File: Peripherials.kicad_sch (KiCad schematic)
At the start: 24 parts, among them J10 IDC_Cable_02x08, J6 Conn_01x02_Pin, J7 USB_C_Receptacle_USB2.0_14P, J8 USB_C_Receptacle_USB2.0_14P, Q1 NMOS, U5 USBLC6-2P6, U6 USBLC6-2P6

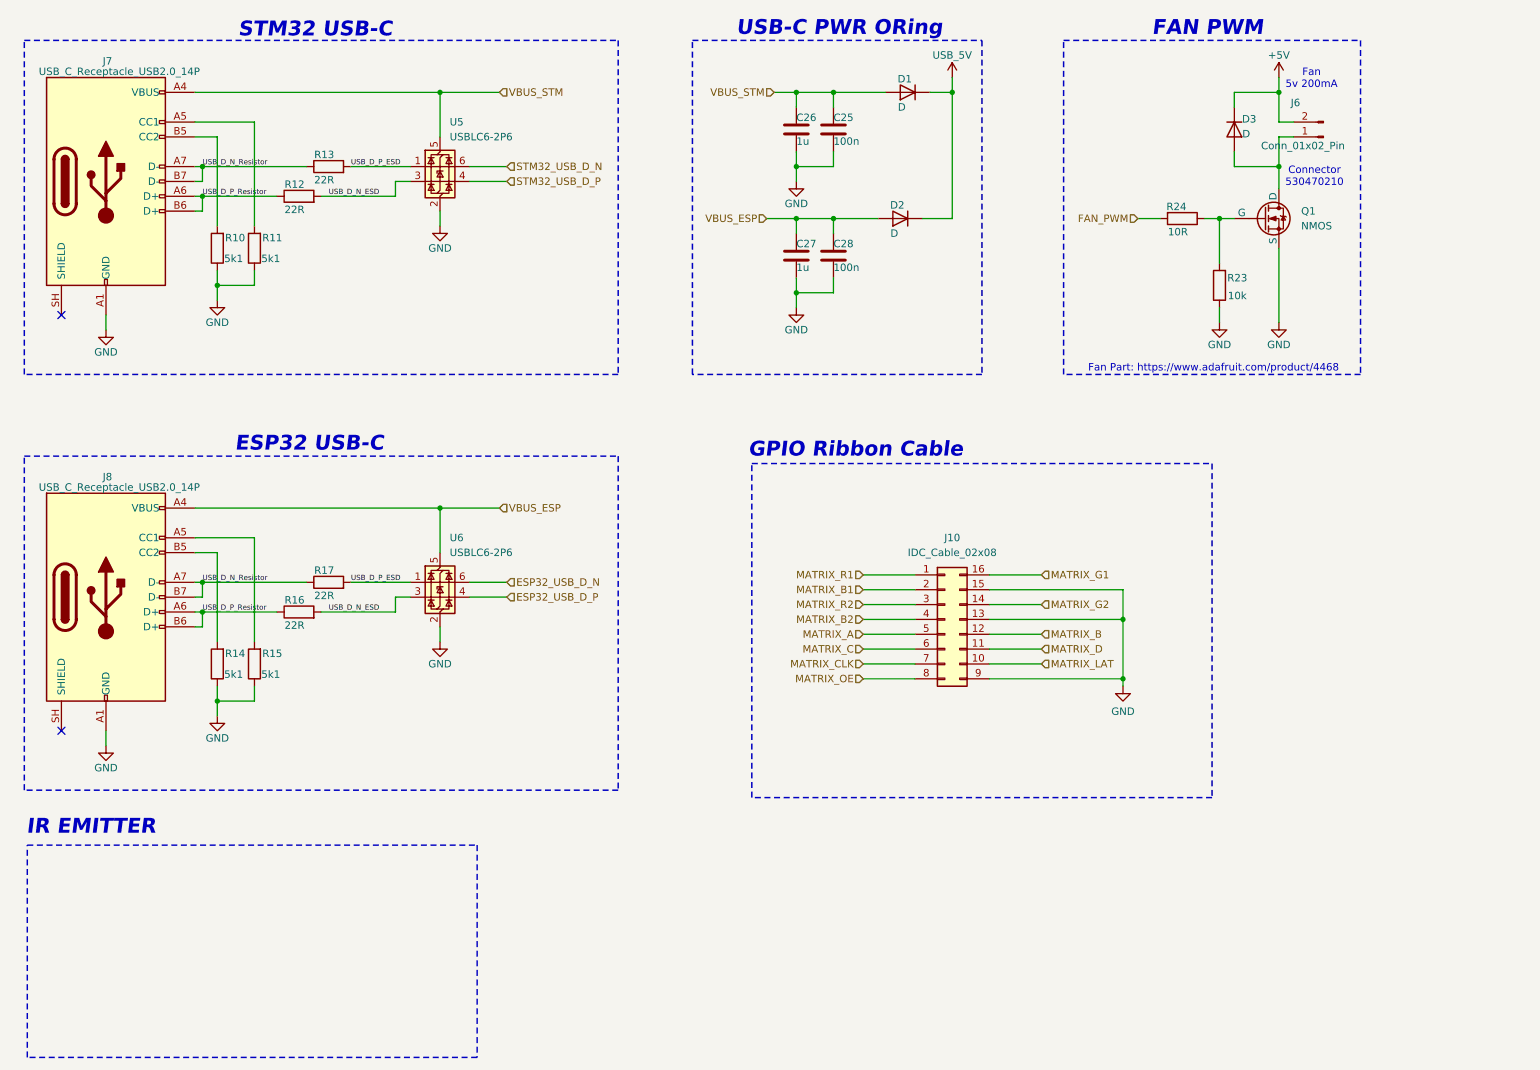
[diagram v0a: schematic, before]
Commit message: Major Changes - Schematic Done??
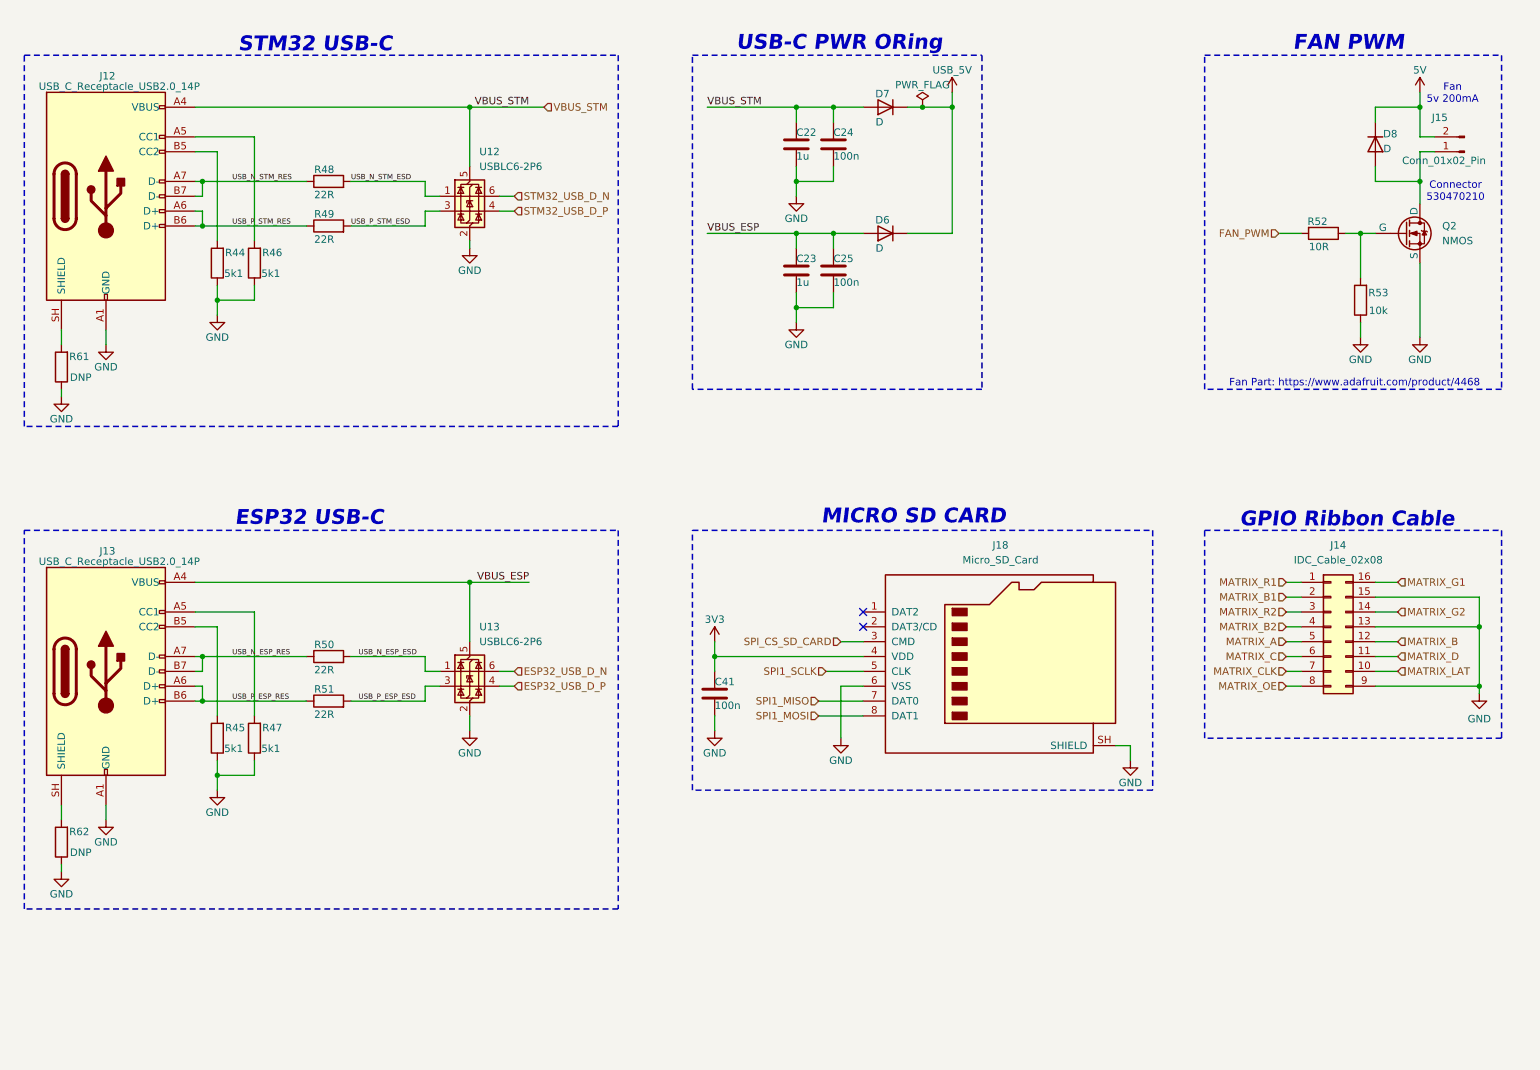
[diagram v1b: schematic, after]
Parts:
- added C41: 100n, Capacitor_SMD:C_0603_1608Metric, symbol Device:C
- added J18: Micro_SD_Card, Connector_Card:microSD_HC_Hirose_DM3BT-DSF-PEJS, symbol Connector:Micro_SD_Card
- added R61, R62: DNP, Resistor_SMD:R_0603_1608Metric, symbol Device:R
- C22: renamed from C26; footprint (none) -> Capacitor_SMD:C_0603_1608Metric
- C23: renamed from C27; footprint (none) -> Capacitor_SMD:C_0603_1608Metric
- C24: renamed from C25; footprint (none) -> Capacitor_SMD:C_0603_1608Metric
- C25: renamed from C28; footprint (none) -> Capacitor_SMD:C_0603_1608Metric
- D6: renamed from D2; footprint Package_TO_SOT_SMD:SOT-666 -> Diode_SMD:D_1206_3216Metric_Pad1.42x1.75mm_HandSolder
- D7: renamed from D1; footprint Package_TO_SOT_SMD:SOT-666 -> Diode_SMD:D_1206_3216Metric_Pad1.42x1.75mm_HandSolder
- D8: renamed from D3; footprint Package_TO_SOT_SMD:SOT-666 -> Diode_SMD:D_0805_2012Metric_Pad1.15x1.40mm_HandSolder
- J12: renamed from J7; footprint (none) -> Connector_USB:USB_C_Receptacle_Palconn_UTC16-G
- J13: renamed from J8; footprint (none) -> Connector_USB:USB_C_Receptacle_Palconn_UTC16-G
- J15: renamed from J6; footprint (none) -> Connector_PinHeader_2.54mm:PinHeader_1x02_P2.54mm_Vertical
- Q2: renamed from Q1; footprint (none) -> Package_TO_SOT_SMD:SOT-23
- R44: renamed from R10; footprint Package_DIP:DIP-8_W7.62mm -> Resistor_SMD:R_0603_1608Metric
- R45: renamed from R14; footprint Package_DIP:DIP-8_W7.62mm -> Resistor_SMD:R_0603_1608Metric
- R46: renamed from R11; footprint Package_DIP:DIP-8_W7.62mm -> Resistor_SMD:R_0603_1608Metric
- R47: renamed from R15; footprint Package_DIP:DIP-8_W7.62mm -> Resistor_SMD:R_0603_1608Metric
- R48: renamed from R13; footprint Package_DIP:DIP-8_W7.62mm -> Resistor_SMD:R_0603_1608Metric
- R49: renamed from R12; footprint Package_DIP:DIP-8_W7.62mm -> Resistor_SMD:R_0603_1608Metric
- R50: renamed from R17; footprint Package_DIP:DIP-8_W7.62mm -> Resistor_SMD:R_0603_1608Metric
- R51: renamed from R16; footprint Package_DIP:DIP-8_W7.62mm -> Resistor_SMD:R_0603_1608Metric
- R52: renamed from R24; footprint Package_DIP:DIP-8_W7.62mm -> Resistor_SMD:R_0603_1608Metric
- R53: renamed from R23; footprint Package_DIP:DIP-8_W7.62mm -> Resistor_SMD:R_0603_1608Metric
- renumbered J10 to J14, U5 to U12, U6 to U13
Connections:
- net GND: now also C41.2, J18.6 (VSS), J18.SH (SHIELD), R61.1, R62.1
- net at J13.SH (SHIELD): now also R62.2
- net at J12.SH (SHIELD): now also R61.2
- net +5V renamed 5V
- net USB_D_N_ESD renamed USB_P_ESP_ESD
- net USB_P_ESP_ESD: no longer R49.2, U12.3 (I/O2)
- net USB_D_N_Resistor renamed USB_N_ESP_RES
- net USB_N_ESP_RES: no longer J12.A7 (D-), J12.B7 (D-), R48.1
- net USB_D_P_ESD renamed USB_N_ESP_ESD
- net USB_N_ESP_ESD: no longer R48.2, U12.1 (I/O1)
- net USB_D_P_Resistor renamed USB_P_ESP_RES
- net USB_P_ESP_RES: no longer J12.A6 (D+), J12.B6 (D+), R49.1
- new net 3V3: C41.1, J18.4 (VDD)
- new net SPI1_MISO: J18.7 (DAT0)
- new net SPI1_MOSI: J18.8 (DAT1)
- new net SPI1_SCLK: J18.5 (CLK)
- new net SPI_CS_SD_CARD: J18.3 (CMD)
- new net USB_N_STM_ESD: R48.2, U12.1 (I/O1)
- new net USB_N_STM_RES: J12.A7 (D-), J12.B7 (D-), R48.1
- new net USB_P_STM_ESD: R49.2, U12.3 (I/O2)
- new net USB_P_STM_RES: J12.A6 (D+), J12.B6 (D+), R49.1
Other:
- note added: "MICRO SD CARD"
- note removed: "IR EMITTER"
- moved on the sheet: C22, C23, C24, C25, D6, D7, D8, J12, J13, J14, J15, Q2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
